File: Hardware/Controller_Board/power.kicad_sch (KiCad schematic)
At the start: 35 parts, among them Q1 DMN2400UFB-7, U2 TPS82084, U3 LT8645S, U4 TPS82084, U5 TPS82084, U6 XT30

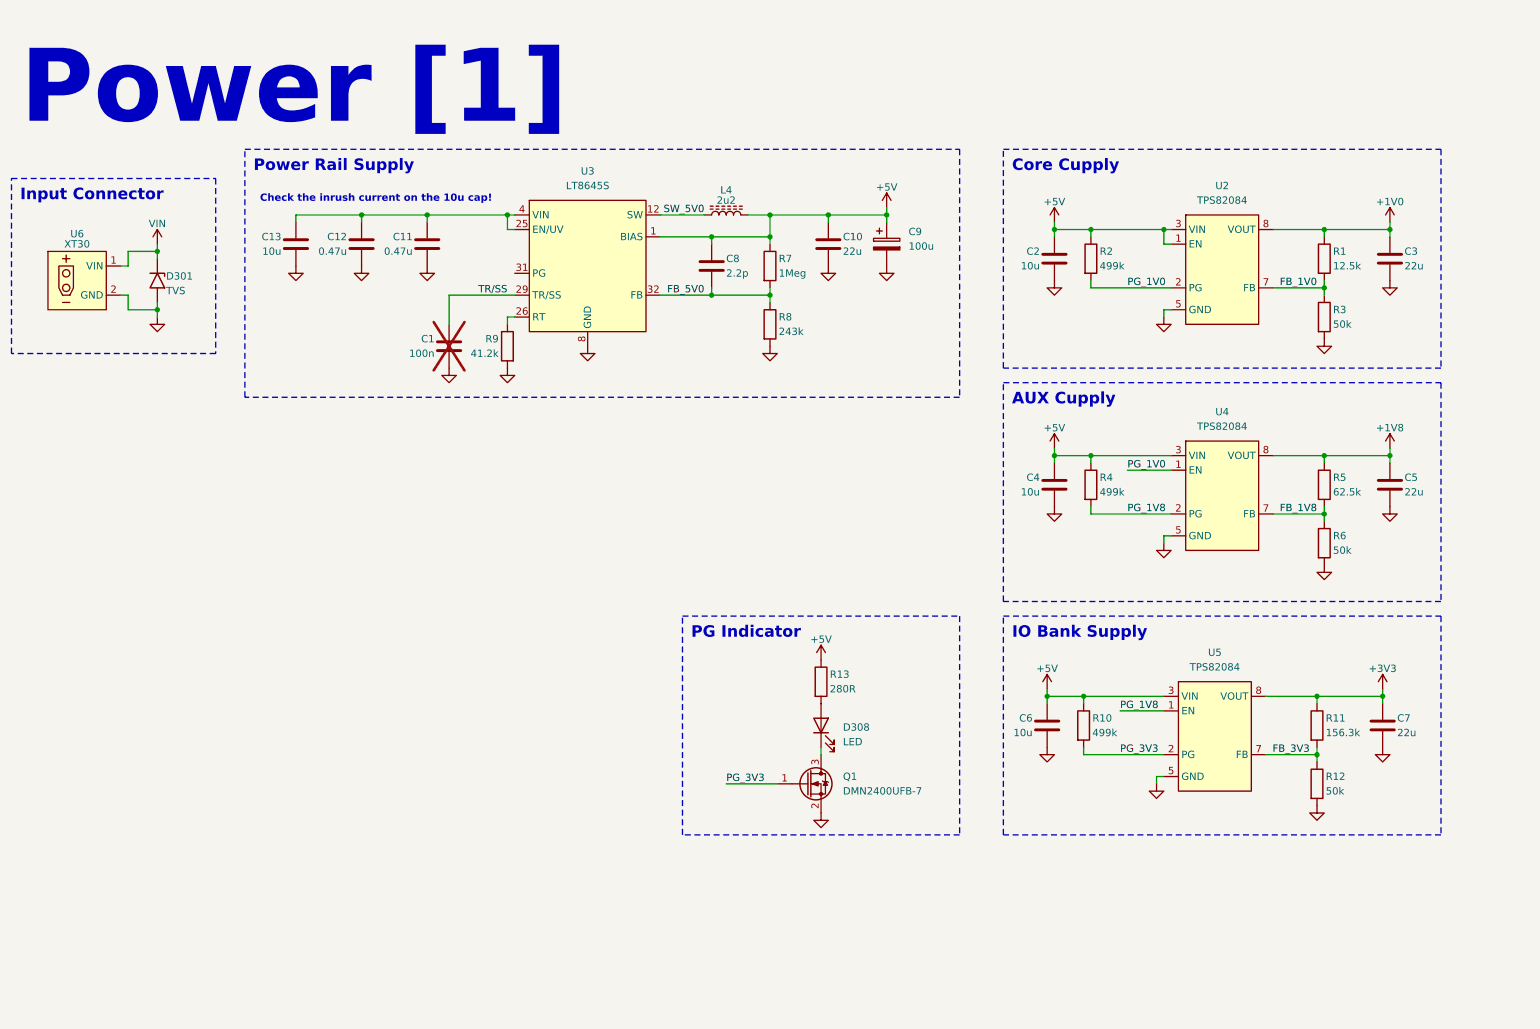
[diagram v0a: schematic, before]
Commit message: Commited Schematic Changes
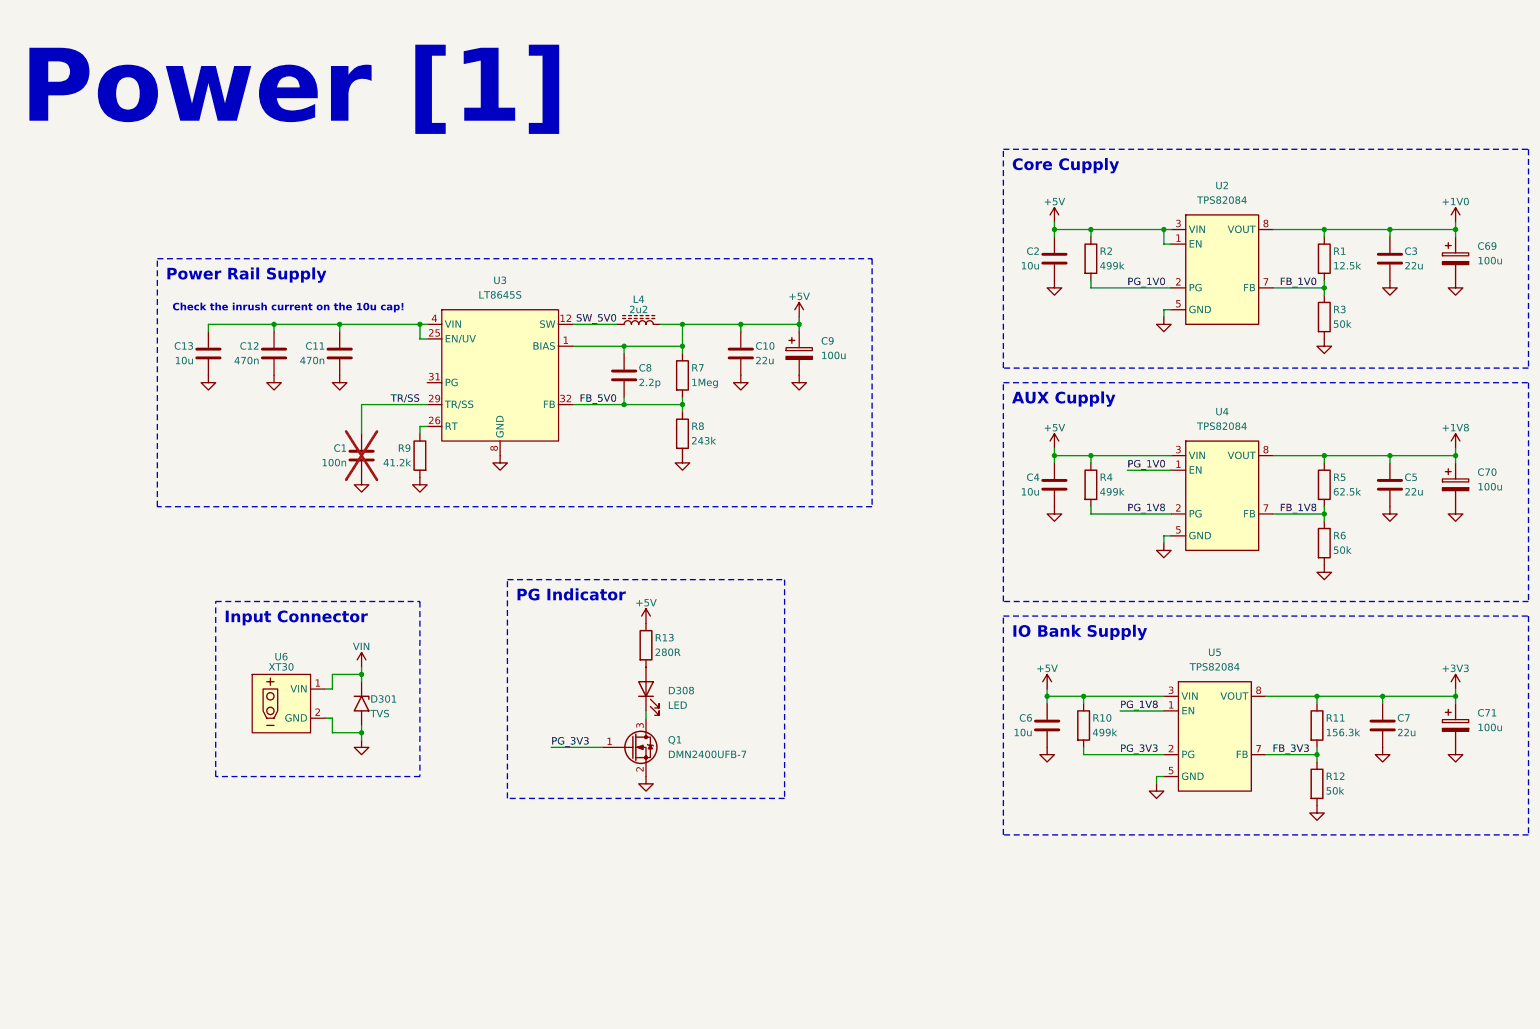
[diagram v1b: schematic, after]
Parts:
- added C69, C70, C71: 100u, Capacitor_SMD:CP_Elec_8x6.5, symbol Device:C_Polarized
- C11, C12: value 0.47u -> 470n
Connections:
- net +1V0: now also C69.1
- net +1V8: now also C70.1
- net +3V3: now also C71.1
- net GND: now also C69.2, C70.2, C71.2
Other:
- moved on the sheet: C1, C10, C11, C12, C13, C8, C9, D301, D308, L4, Q1, R13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

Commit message: Commited Schematic Changes
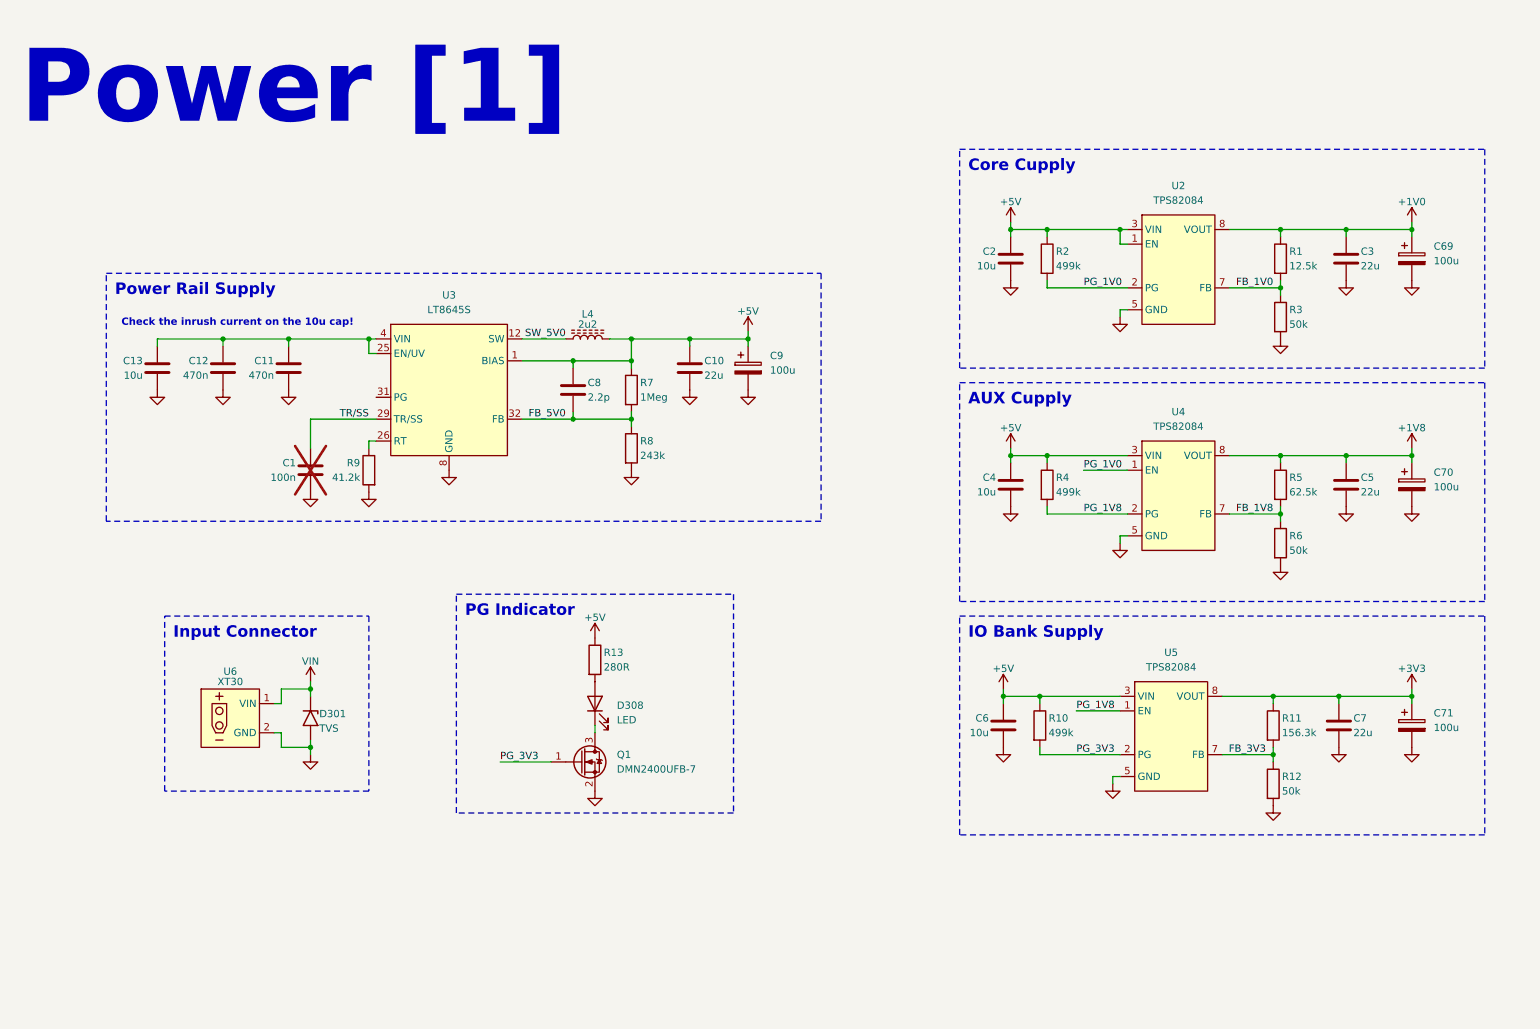
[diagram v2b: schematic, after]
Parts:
- D301: footprint Diode_SMD:D_0402_1005Metric -> (none)
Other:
- moved on the sheet: C1, C10, C11, C12, C13, C2, C3, C4, C5, C6, C69, C7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

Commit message: Updated schematic diagram with configuration
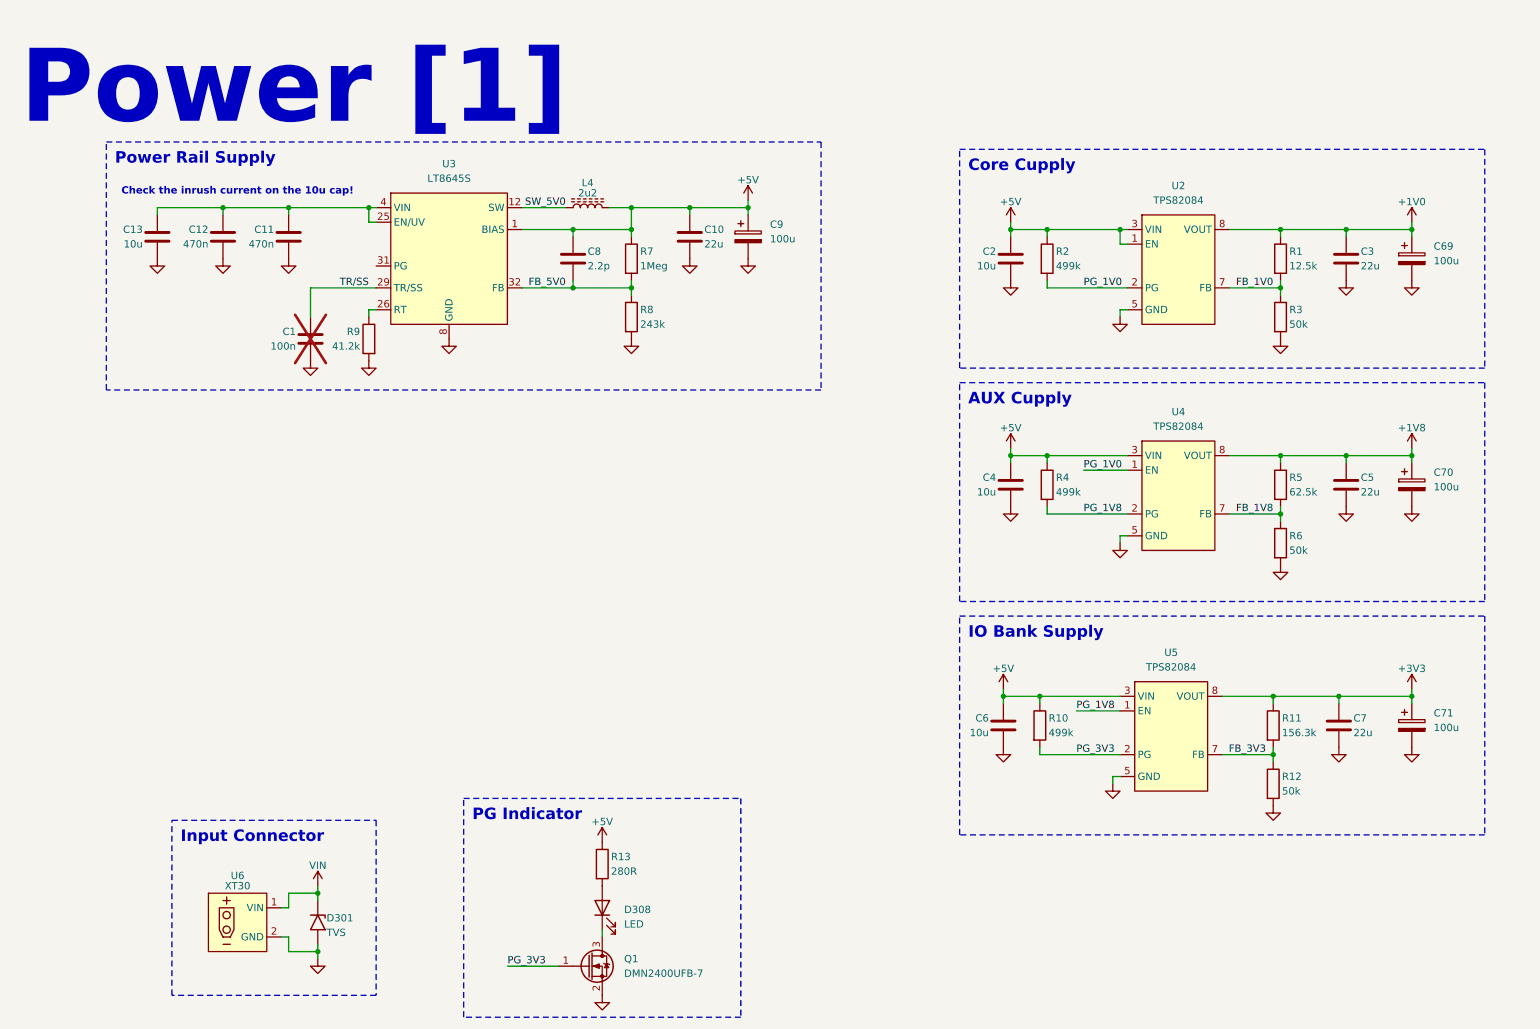
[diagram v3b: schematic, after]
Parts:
- L4: footprint Inductor_SMD:L_Coilcraft_XAL6060-XXX -> Inductor_SMD:L_Coilcraft_XAL6030-XXX
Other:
- moved on the sheet: C1, C10, C11, C12, C13, C8, C9, D301, D308, L4, Q1, R13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
